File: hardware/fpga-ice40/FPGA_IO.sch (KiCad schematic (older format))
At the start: 1 part, among them U1 iCE40HX4K-TQ144

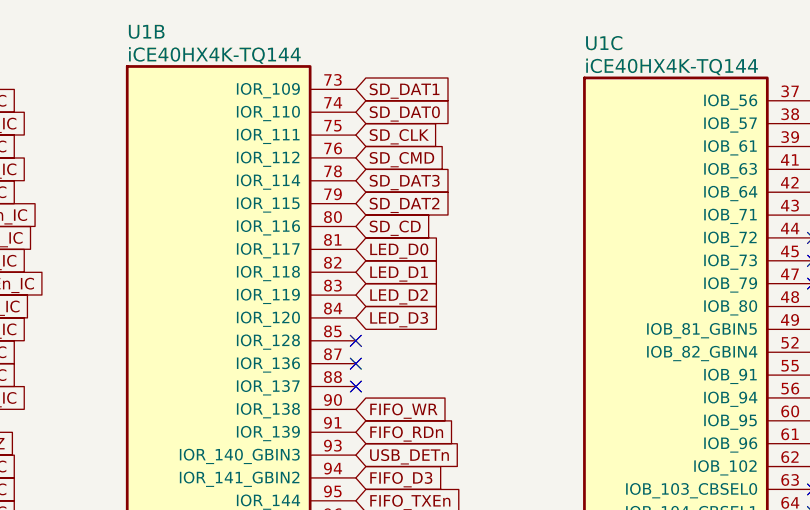
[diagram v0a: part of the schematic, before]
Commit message: Completed verification of all pins for all symbols
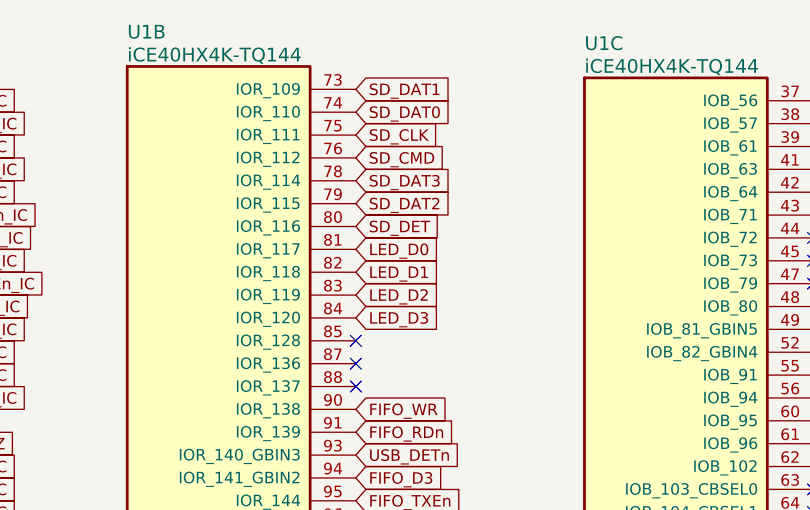
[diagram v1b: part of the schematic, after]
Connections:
- net SD_CD renamed SD_DET
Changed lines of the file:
@@
 LED_D0
 Text GLabel 4850 3400 2    50   Input ~ 0
-SD_CD
+SD_DET
 Text GLabel 4850 3300 2    50   Input ~ 0
 SD_DAT2
